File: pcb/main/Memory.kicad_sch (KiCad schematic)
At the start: 5 parts, among them U7 SST26VF064B

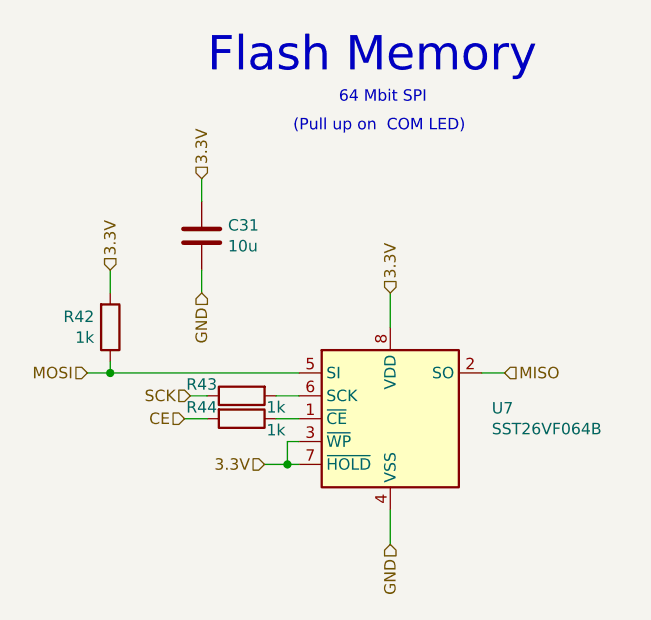
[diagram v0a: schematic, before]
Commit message: feat: updated BOM information
Some components are still without MNF and Seller information
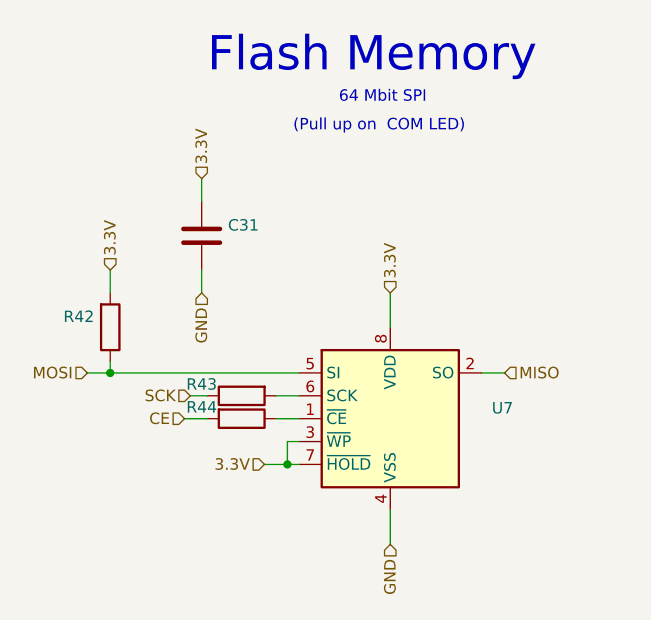
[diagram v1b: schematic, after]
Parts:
- C31: value 10u -> (none); footprint Capacitor_SMD:C_0805_2012Metric_Pad1.18x1.45mm_HandSolder -> (none)
- R42, R43, R44: value 1k -> (none); footprint Resistor_SMD:R_0805_2012Metric_Pad1.15x1.40mm_HandSolder -> (none); MFN (none) -> KOA Speer; MFP (none) -> RK73H2ATTD1001F; S1PL (none) -> https://www.mouser.com/ProductDetail/KOA-Speer/RK73H2ATTD10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; S1PN (none) -> 660-RK73H2ATTD1001F
- U7: value SST26VF064B -> (none); footprint Package_SO:SOIJ-8_5.3x5.3mm_P1.27mm -> (none)
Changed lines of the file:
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@@
     (in_bom yes) (on_board yes)
     (property "Reference" "R44" (id 0) (at 112.395 57.785 90))
-    (property "Value" "1k" (id 1) (at 120.65 60.325 90))
-    (property "Footprint" "Resistor_SMD:R_0805_2012Metric_Pad1.15x1.40mm_HandSolder" (id 2) (at 116.84 57.277 90)
+    (property "Value" "" (id 1) (at 120.65 60.325 90))
+    (property "Footprint" "" (id 2) (at 116.84 57.277 90)
       (effects (font (size 1.27 1.27)) hide)
     )
-    (property "Datasheet" "~" (id 3) (at 116.84 59.055 0)
+    (property "Datasheet" "https://www.mouser.com/datasheet/2/219/RK73H-1825326.pdf" (id 3) (at 116.84 59.055 0)
+      (effects (font (size 1.27 1.27)) hide)
+    )
+    (property "Description" "Thick Film Resistors - SMD 1/4watts 1Kohms 1% " (id 4) (at 116.84 59.055 0)
+      (effects (font (size 1.27 1.27)) hide)
+    )
+    (property "MFN" "KOA Speer " (id 5) (at 116.84 59.055 0)
+      (effects (font (size 1.27 1.27)) hide)
+    )
+    (property "MFP" "RK73H2ATTD1001F " (id 6) (at 116.84 59.055 0)
+      (effects (font (size 1.27 1.27)) hide)
+    )
+    (property "S1PL" "https://www.mouser.com/ProductDetail/KOA-Speer/RK73H2ATTD1001F?qs=sGAEpiMZZMtlubZbdhIBIHMXi0pPDQ96wRIUy6HwZNc%3D" (id 7) (at 116.84 59.055 0)
+      (effects (font (size 1.27 1.27)) hide)
+    )
+    (property "S1PN" "660-RK73H2ATTD1001F " (id 8) (at 116.84 59.055 0)
       (effects (font (size 1.27 1.27)) hide)
     )
@@
     (in_bom yes) (on_board yes)
     (property "Reference" "R43" (id 0) (at 112.395 55.245 90))
-    (property "Value" "1k" (id 1) (at 120.65 57.785 90))
-    (property "Footprint" "Resistor_SMD:R_0805_2012Metric_Pad1.15x1.40mm_HandSolder" (id 2) (at 116.84 54.737 90)
+    (property "Value" "" (id 1) (at 120.65 57.785 90))
+    (property "Footprint" "" (id 2) (at 116.84 54.737 90)
       (effects (font (size 1.27 1.27)) hide)
     )
-    (property "Datasheet" "~" (id 3) (at 116.84 56.515 0)
+    (property "Datasheet" "https://www.mouser.com/datasheet/2/219/RK73H-1825326.pdf" (id 3) (at 116.84 56.515 0)
+      (effects (font (size 1.27 1.27)) hide)
+    )
+    (property "Description" "Thick Film Resistors - SMD 1/4watts 1Kohms 1% " (id 4) (at 116.84 56.515 0)
+      (effects (font (size 1.27 1.27)) hide)
+    )
+    (property "MFN" "KOA Speer " (id 5) (at 116.84 56.515 0)
+      (effects (font (size 1.27 1.27)) hide)
+    )
+    (property "MFP" "RK73H2ATTD1001F " (id 6) (at 116.84 56.515 0)
+      (effects (font (size 1.27 1.27)) hide)
+    )
+    (property "S1PL" "https://www.mouser.com/ProductDetail/KOA-Speer/RK73H2ATTD1001F?qs=sGAEpiMZZMtlubZbdhIBIHMXi0pPDQ96wRIUy6HwZNc%3D" (id 7) (at 116.84 56.515 0)
+      (effects (font (size 1.27 1.27)) hide)
+    )
+    (property "S1PN" "660-RK73H2ATTD1001F " (id 8) (at 116.84 56.515 0)
       (effects (font (size 1.27 1.27)) hide)
     )
@@
       (effects (font (size 1.27 1.27)) (justify right))
     )
-    (property "Value" "1k" (id 1) (at 100.457 50.038 0)
+    (property "Value" "" (id 1) (at 100.457 50.038 0)
       (effects (font (size 1.27 1.27)) (justify right))
     )
-    (property "Footprint" "Resistor_SMD:R_0805_2012Metric_Pad1.15x1.40mm_HandSolder" (id 2) (at 100.457 48.895 90)
+    (property "Footprint" "" (id 2) (at 100.457 48.895 90)
       (effects (font (size 1.27 1.27)) hide)
     )
-    (property "Datasheet" "~" (id 3) (at 102.235 48.895 0)
+    (property "Datasheet" "https://www.mouser.com/datasheet/2/219/RK73H-1825326.pdf" (id 3) (at 102.235 48.895 0)
+      (effects (font (size 1.27 1.27)) hide)
+    )
+    (property "Description" "Thick Film Resistors - SMD 1/4watts 1Kohms 1% " (id 4) (at 102.235 48.895 0)
+      (effects (font (size 1.27 1.27)) hide)
+    )
+    (property "MFN" "KOA Speer " (id 5) (at 102.235 48.895 0)
+      (effects (font (size 1.27 1.27)) hide)
+    )
+    (property "MFP" "RK73H2ATTD1001F " (id 6) (at 102.235 48.895 0)
+      (effects (font (size 1.27 1.27)) hide)
+    )
+    (property "S1PL" "https://www.mouser.com/ProductDetail/KOA-Speer/RK73H2ATTD1001F?qs=sGAEpiMZZMtlubZbdhIBIHMXi0pPDQ96wRIUy6HwZNc%3D" (id 7) (at 102.235 48.895 0)
+      (effects (font (size 1.27 1.27)) hide)
+    )
+    (property "S1PN" "660-RK73H2ATTD1001F " (id 8) (at 102.235 48.895 0)
       (effects (font (size 1.27 1.27)) hide)
     )
@@
       (effects (font (size 1.27 1.27)) (justify left))
     )
-    (property "Value" "10u" (id 1) (at 115.316 39.878 0)
+    (property "Value" "" (id 1) (at 115.316 39.878 0)
       (effects (font (size 1.27 1.27)) (justify left))
     )
-    (property "Footprint" "Capacitor_SMD:C_0805_2012Metric_Pad1.18x1.45mm_HandSolder" (id 2) (at 113.3602 42.545 0)
+    (property "Footprint" "" (id 2) (at 113.3602 42.545 0)
       (effects (font (size 1.27 1.27)) hide)
     )
@@
       (effects (font (size 1.27 1.27)) (justify left))
     )
-    (property "Value" "SST26VF064B" (id 1) (at 144.6276 60.198 0)
+    (property "Value" "" (id 1) (at 144.6276 60.198 0)
       (effects (font (size 1.27 1.27)) (justify left))
     )
-    (property "Footprint" "Package_SO:SOIJ-8_5.3x5.3mm_P1.27mm" (id 2) (at 133.35 76.835 0)
+    (property "Footprint" "" (id 2) (at 133.35 76.835 0)
       (effects (font (size 1.27 1.27)) hide)
     )

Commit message: feat: updated BOM
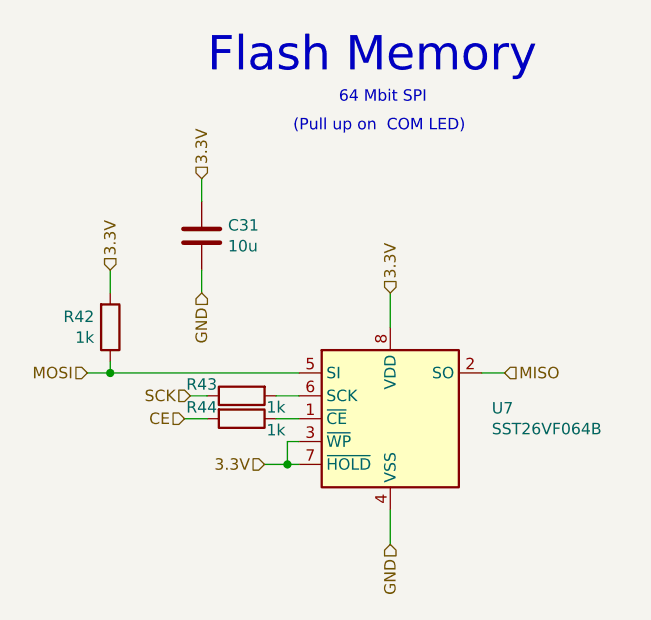
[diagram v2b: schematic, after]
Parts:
- C31: value (none) -> 10u; footprint (none) -> Capacitor_SMD:C_0805_2012Metric_Pad1.18x1.45mm_HandSolder
- R42, R43, R44: value (none) -> 1k
- U7: value (none) -> SST26VF064B
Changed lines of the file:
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@@
     (in_bom yes) (on_board yes)
     (property "Reference" "R44" (id 0) (at 112.395 57.785 90))
-    (property "Value" "" (id 1) (at 120.65 60.325 90))
+    (property "Value" "1k" (id 1) (at 120.65 60.325 90))
     (property "Footprint" "" (id 2) (at 116.84 57.277 90)
       (effects (font (size 1.27 1.27)) hide)
@@
     (in_bom yes) (on_board yes)
     (property "Reference" "R43" (id 0) (at 112.395 55.245 90))
-    (property "Value" "" (id 1) (at 120.65 57.785 90))
+    (property "Value" "1k" (id 1) (at 120.65 57.785 90))
     (property "Footprint" "" (id 2) (at 116.84 54.737 90)
       (effects (font (size 1.27 1.27)) hide)
@@
       (effects (font (size 1.27 1.27)) (justify right))
     )
-    (property "Value" "" (id 1) (at 100.457 50.038 0)
+    (property "Value" "1k" (id 1) (at 100.457 50.038 0)
       (effects (font (size 1.27 1.27)) (justify right))
     )
@@
       (effects (font (size 1.27 1.27)) (justify left))
     )
-    (property "Value" "" (id 1) (at 115.316 39.878 0)
+    (property "Value" "10u" (id 1) (at 115.316 39.878 0)
       (effects (font (size 1.27 1.27)) (justify left))
     )
-    (property "Footprint" "" (id 2) (at 113.3602 42.545 0)
+    (property "Footprint" "Capacitor_SMD:C_0805_2012Metric_Pad1.18x1.45mm_HandSolder" (id 2) (at 113.3602 42.545 0)
       (effects (font (size 1.27 1.27)) hide)
     )
@@
       (effects (font (size 1.27 1.27)) (justify left))
     )
-    (property "Value" "" (id 1) (at 144.6276 60.198 0)
+    (property "Value" "SST26VF064B" (id 1) (at 144.6276 60.198 0)
       (effects (font (size 1.27 1.27)) (justify left))
     )
